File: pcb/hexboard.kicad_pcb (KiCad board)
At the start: 2 copper layers, 121.4 x 97.6 mm, 43 parts, among them J1 Conn_01x02_Pin, SW1 SW_Push_45deg, SW10 SW_Push_45deg, SW11 SW_Push_45deg, SW12 SW_Push_45deg, SW13 SW_Push_45deg, SW14 SW_Push_45deg, SW15 SW_Push_45deg, SW16 SW_Push_45deg, SW17 SW_Push_45deg, SW18 SW_Push_45deg, SW19 SW_SPDT, SW2 SW_Push_45deg, SW3 SW_Push_45deg, SW4 SW_Push_45deg, SW5 SW_Push_45deg, SW6 SW_Push_45deg, SW7 SW_Push_45deg, SW8 SW_Push_45deg, SW9 SW_Push_45deg, U2 XIAO-nRF52840-SMD

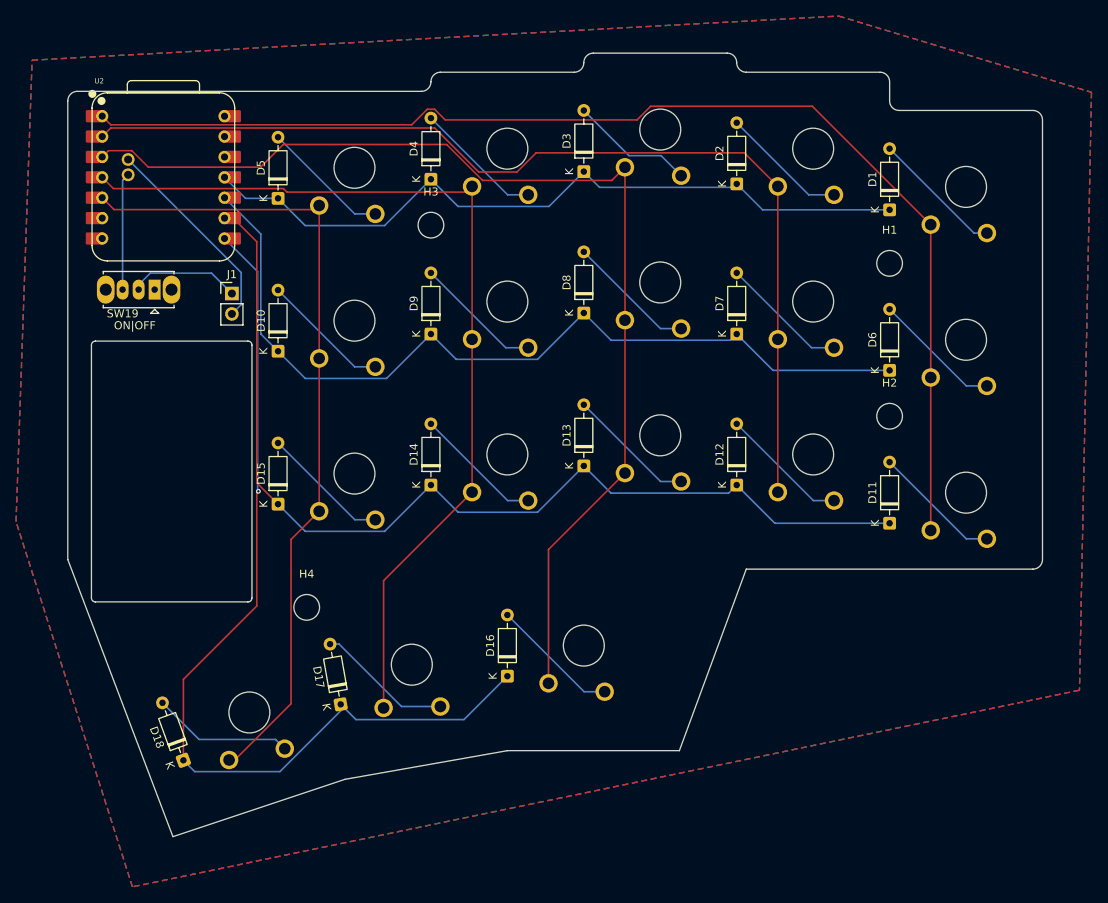
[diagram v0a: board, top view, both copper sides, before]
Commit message: Updated PCB
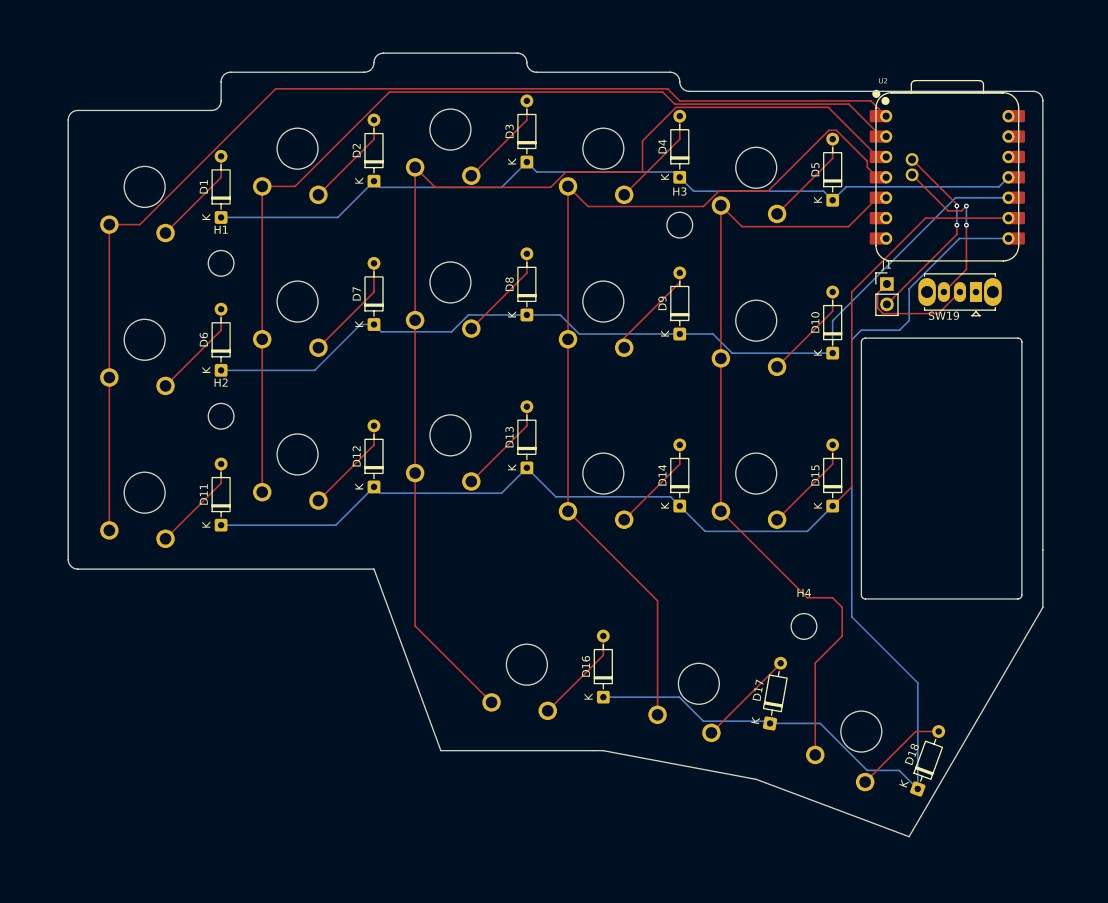
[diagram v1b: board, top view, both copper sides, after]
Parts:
- moved SW1 102.3 mm to (56.8, 52.5)
- moved SW11 102.3 mm to (56.8, 90.5)
- moved SW6 102.3 mm to (56.8, 71.5)
- moved SW19 102.3 mm to (160.4, 65.5)
- moved U2 97.7 mm to (156.8, 51.3)
- moved D18 91.6 mm to (153.1, 127.5), turned to 70 degrees
- moved D1 83.3 mm to (66.3, 56.3)
- moved D11 83.3 mm to (66.3, 94.6)
- moved D6 83.3 mm to (66.3, 75.3)
- moved H1 83.3 mm to (66.3, 62.0)
- moved H2 83.3 mm to (66.3, 81.0)
- moved J1 81.6 mm to (149.3, 64.5)
- moved SW18 76.3 mm to (146.1, 120.3), turned to -20 degrees
- moved D10 69.1 mm to (142.5, 73.2)
- moved D15 69.1 mm to (142.5, 92.2)
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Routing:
- net Row 3: track 118.6 -> 130.4 mm, vias 1 -> 0
- net Row 0: track 93.3 -> 104.8 mm
- net Row 2: track 126.6 -> 135.4 mm
- net Column 0: track 149.9 -> 143.3 mm
- net B+: track 14.6 -> 20.8 mm, vias 0 -> 2
- net Net-(D18-A): track 17.6 -> 11.8 mm
- net Row 1: track 109.1 -> 114.1 mm
- net Net-(D17-A): track 17.0 -> 12.2 mm
- net Column 1: track 127.7 -> 123.0 mm
- net Net-(D1-A): track 16.5 -> 12.4 mm
- net Net-(D5-A): track 16.1 -> 12.2 mm
- net Net-(D10-A): track 16.1 -> 12.2 mm
- net Net-(D11-A): track 16.1 -> 12.2 mm
- net Net-(D15-A): track 16.1 -> 12.2 mm
- net Net-(D12-A): track 16.1 -> 12.2 mm
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- removed copper zone on B.Cu, net (none)
- removed copper zone on F.Cu, net (none)
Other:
- outline, holes or cut-outs redrawn
- board text removed: "+ -"
- board text removed: "ON|OFF"
